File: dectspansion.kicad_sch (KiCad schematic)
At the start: 21 parts, among them J1 Hexpansion-Connector, J2 Conn_02x10_Odd_Even, J3 AudioJack4, U2 SC14CVMDECT

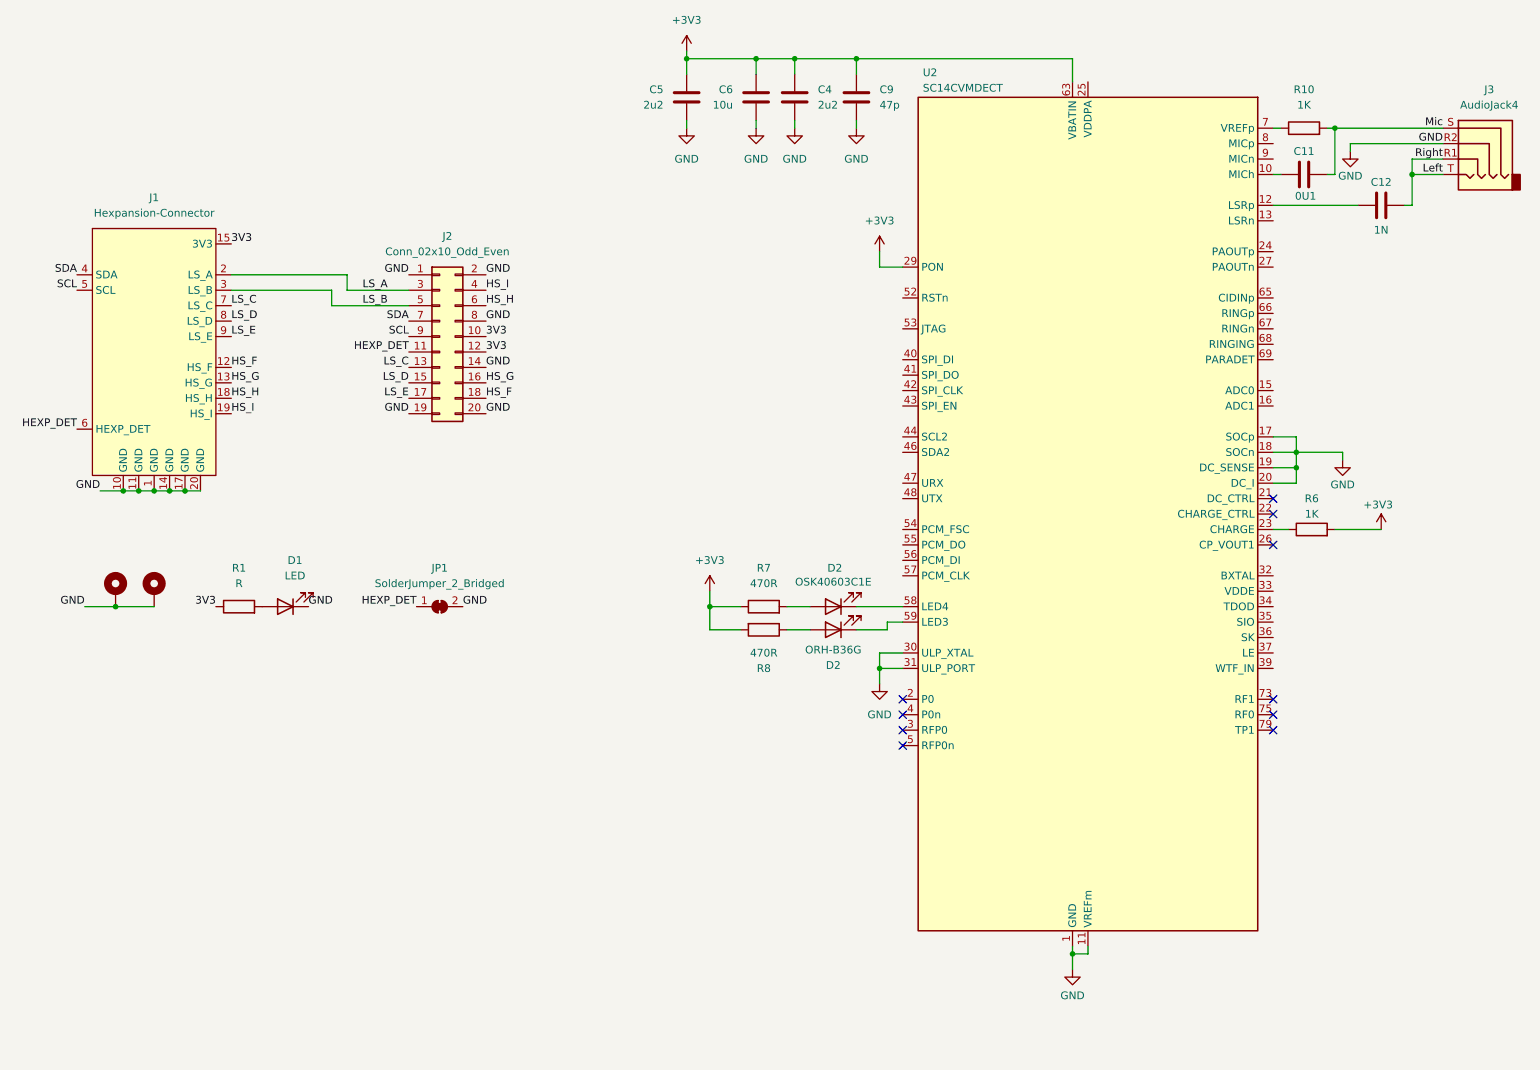
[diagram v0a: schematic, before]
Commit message: Created PCB layout
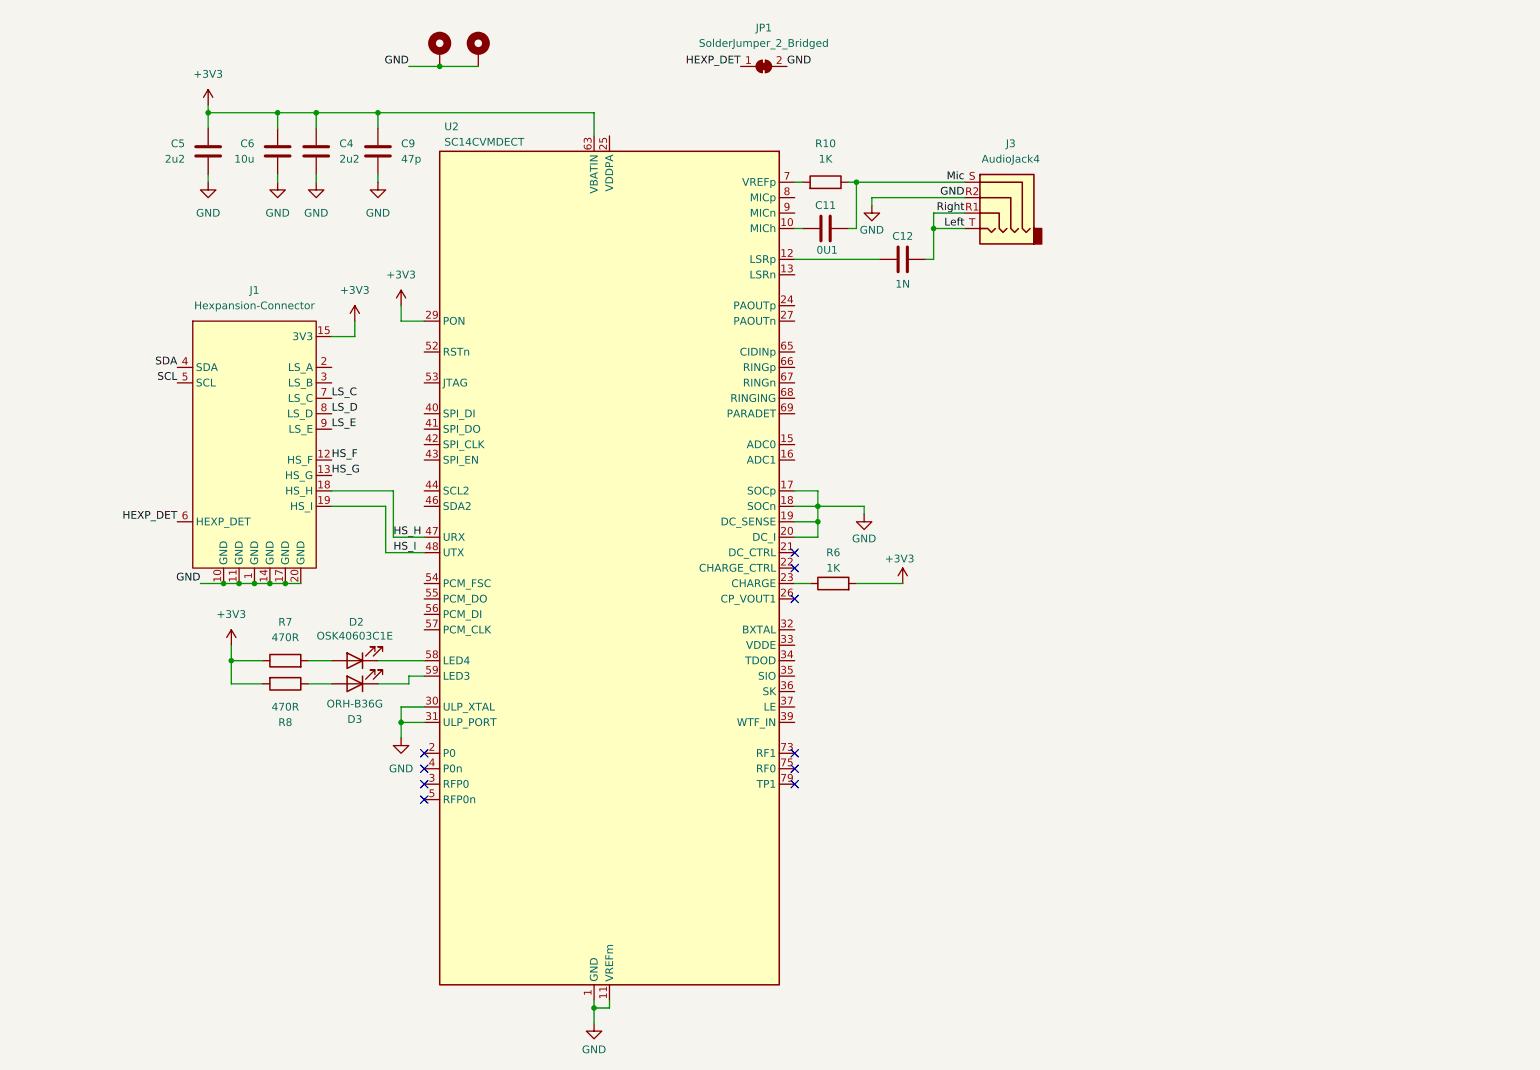
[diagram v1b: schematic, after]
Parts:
- removed D1: LED, LED_SMD:LED_0805_2012Metric, symbol Device:LED
- removed J2: Conn_02x10_Odd_Even, Connector_PinHeader_2.54mm:PinHeader_2x10_P2.54mm_Vertical, symbol Connector_Generic:Conn_02x10_Odd_Even
- removed R1: R, Resistor_SMD:R_0603_1608Metric, symbol Device:R
- renumbered D2 to D3
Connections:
- net 3V3 is gone; now on net +3V3: J1.15 (3V3), J1.16 (3V3)
- net HS_H: now also U2.47 (URX)
- net HS_I: now also U2.48 (UTX)
- net Mic: now also R10.1; no longer R10.2
- net at U2.7 (VREFp): now also R10.2; no longer R10.1
- net LS_A: no longer names the net of J1.2 (LS_A)
- net LS_B: no longer names the net of J1.3 (LS_B)
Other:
- moved on the sheet: C11, C12, C4, C5, C6, C9, D2, D3, J1, J3, JP1, R10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

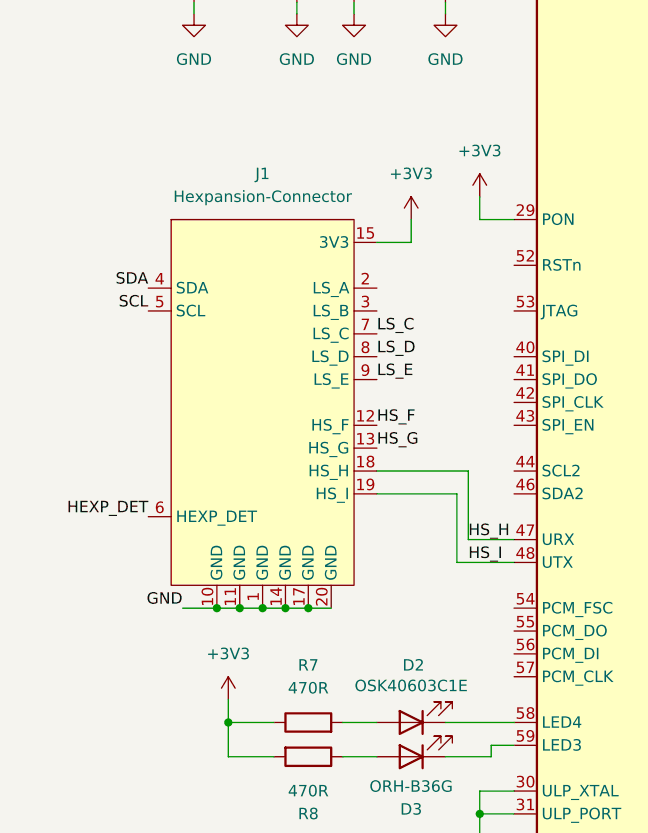
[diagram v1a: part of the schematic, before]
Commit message: Created PCB layout
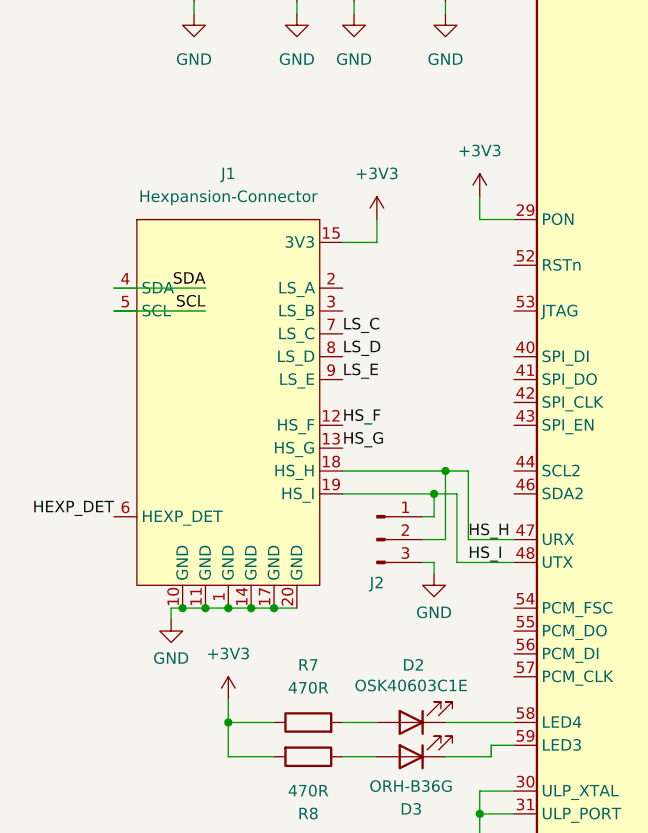
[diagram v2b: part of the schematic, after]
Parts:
- added J2: Conn_01x03_Pin, Connector_PinHeader_2.54mm:PinHeader_1x03_P2.54mm_Vertical, symbol Connector:Conn_01x03_Pin
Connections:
- net GND: now also J2.3 (Pin_3)
- net HS_H: now also J2.2 (Pin_2)
- net HS_I: now also J2.1 (Pin_1)
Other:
- moved on the sheet: J1
